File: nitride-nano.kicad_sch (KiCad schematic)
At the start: 7 parts, among them J3 Conn_01x04_Pin, J6 Conn_01x04_Pin

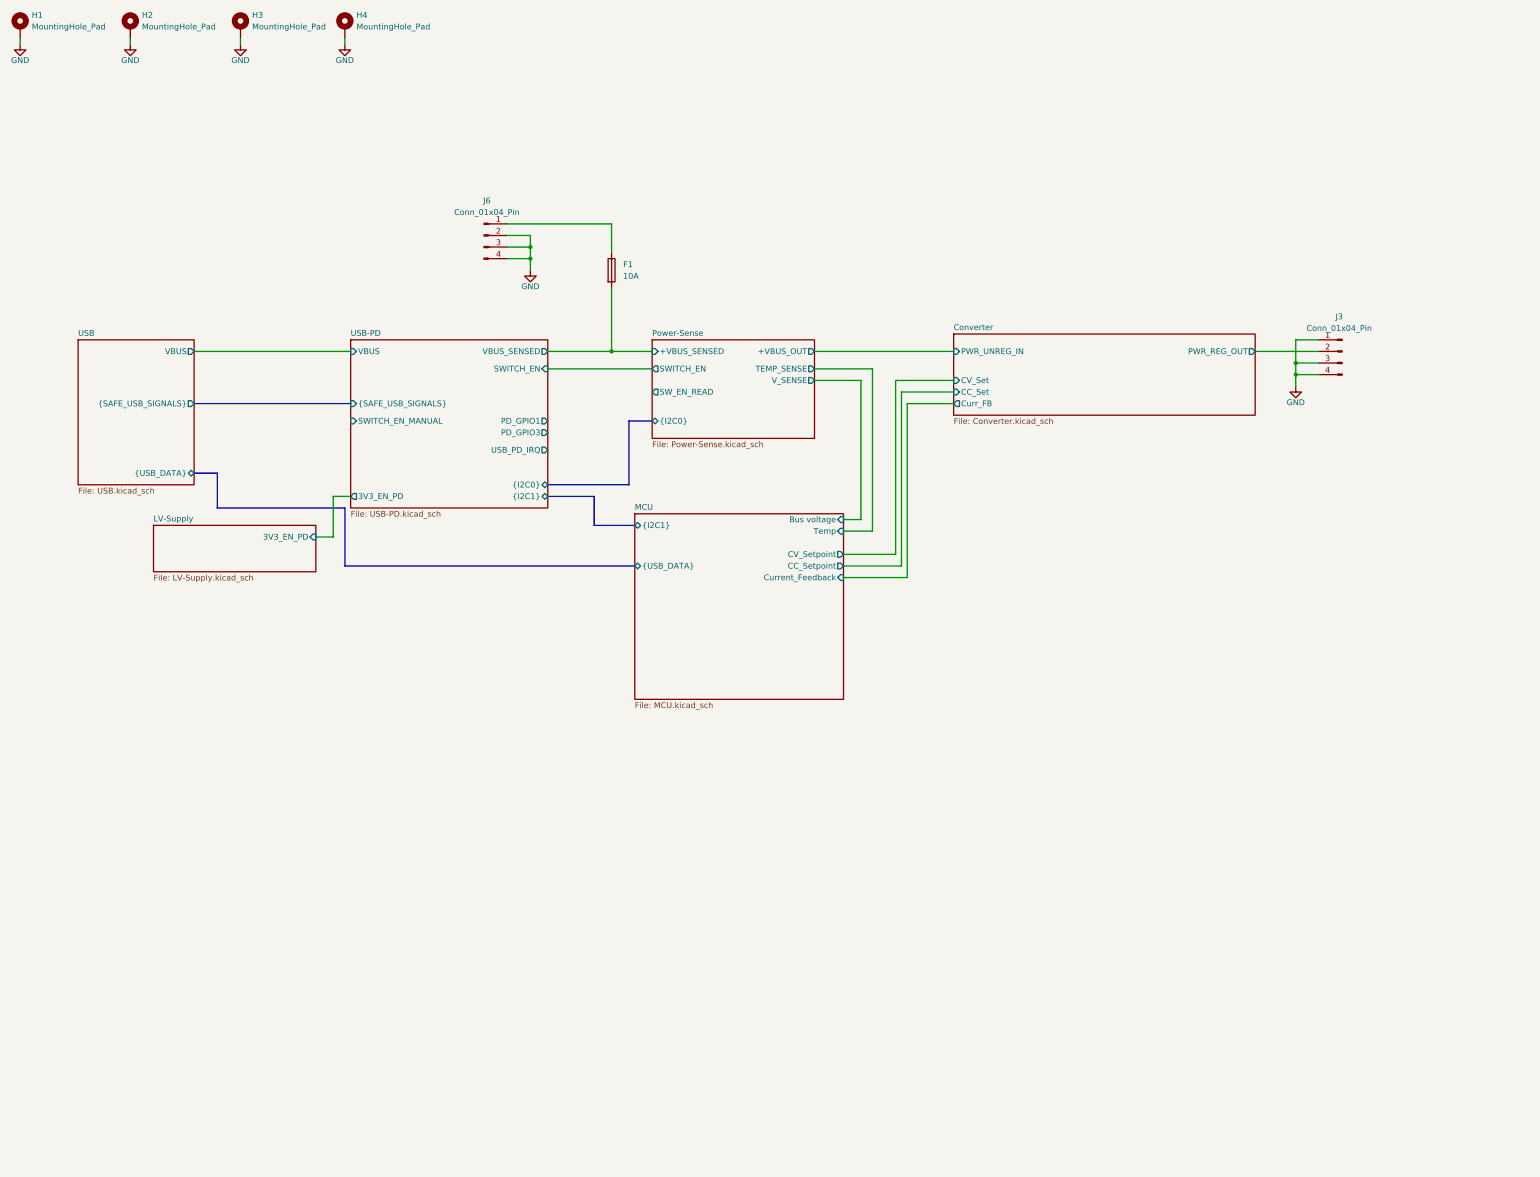
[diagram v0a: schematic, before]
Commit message: Finished layout
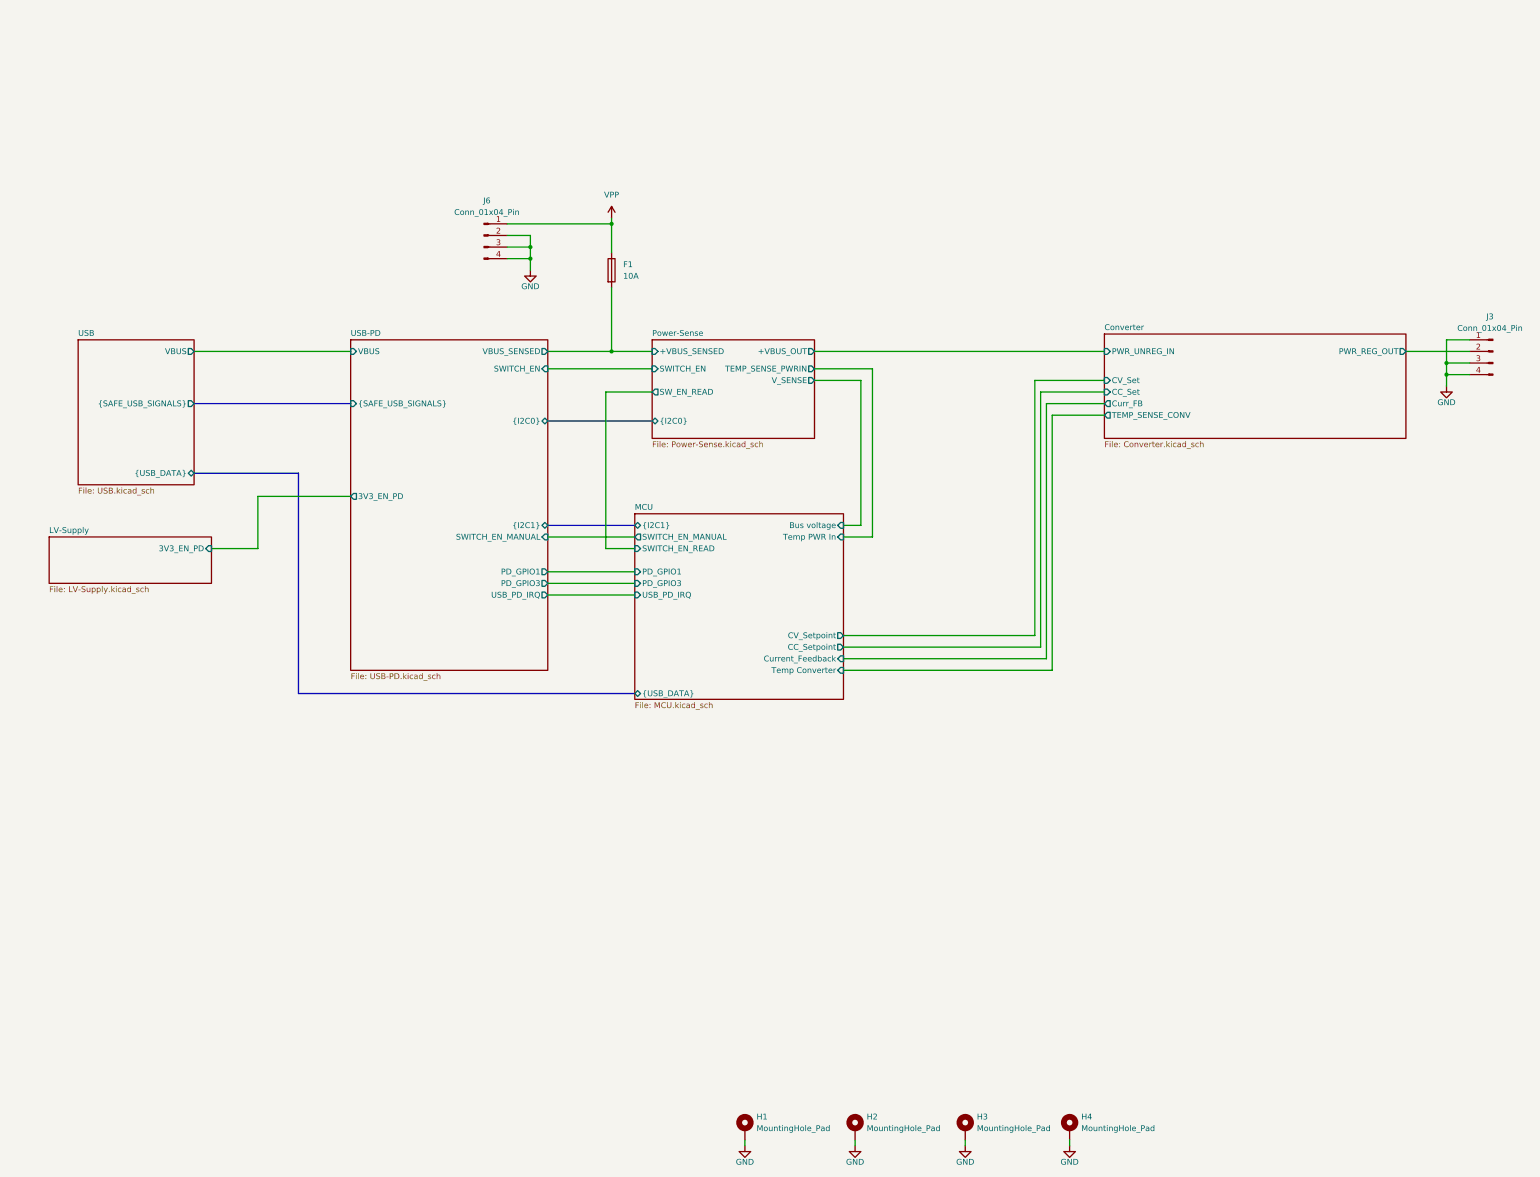
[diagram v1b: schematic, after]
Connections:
- net VPP: now reaches F1.1, J6.1 (Pin_1)
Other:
- sheet Converter ports: added TEMP_SENSE_CONV; removed none
- sheet MCU ports: added PD_GPIO1, PD_GPIO3, SWITCH_EN_MANUAL, SWITCH_EN_READ, Temp Converter, Temp PWR In, USB_PD_IRQ; removed Temp
- sheet Power-Sense ports: added TEMP_SENSE_PWRIN; removed TEMP_SENSE
- moved on the sheet: H1, H2, H3, H4, J3
